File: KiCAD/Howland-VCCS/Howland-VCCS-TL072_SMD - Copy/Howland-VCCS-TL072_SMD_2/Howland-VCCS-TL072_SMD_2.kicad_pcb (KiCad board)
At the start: 2 copper layers, 24.5 x 25.4 mm, 16 parts, among them J1 Conn_01x03_Pin, J2 Conn_01x03_Pin, U1 TL072

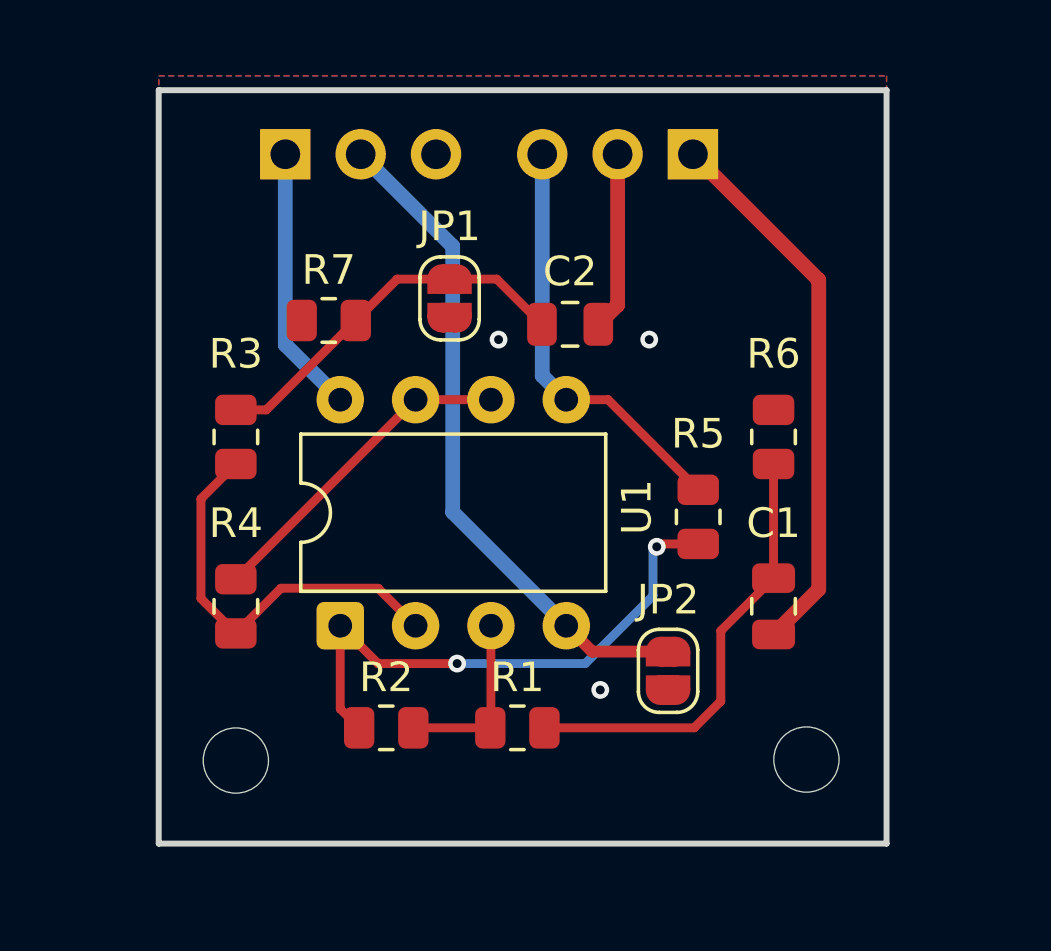
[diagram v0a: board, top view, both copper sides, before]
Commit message: Add Project Folder: KICAD
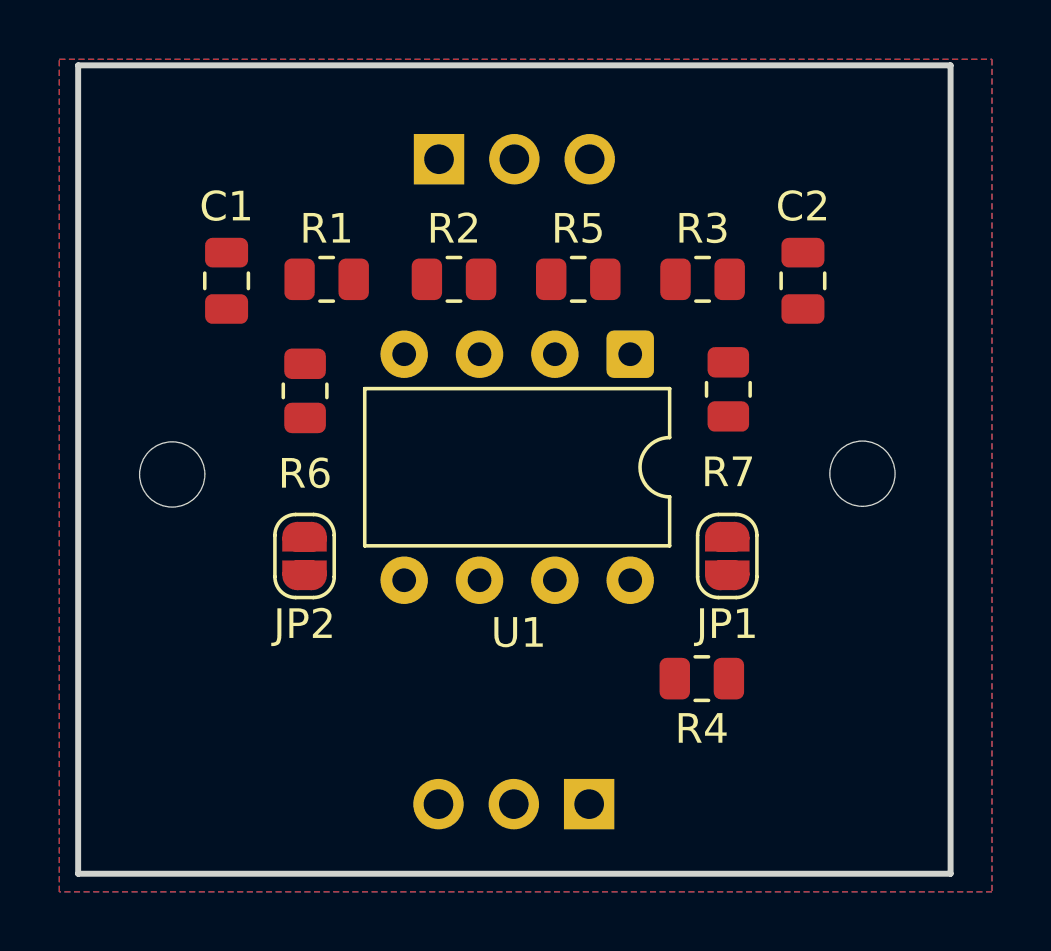
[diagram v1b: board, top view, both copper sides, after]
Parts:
- moved J2 24.2 mm to (192.4, 105.1), turned to 90 degrees
- moved C1 21.5 mm to (180.2, 87.4), turned to -90 degrees
- moved R3 16.6 mm to (196.2, 87.4), turned to 180 degrees
- moved R1 16.4 mm to (183.6, 87.4), turned to 0 degrees
- moved R4 15.9 mm to (196.2, 100.8), turned to 180 degrees
- moved R6 15.9 mm to (182.8, 91.1), turned to 90 degrees
- moved R2 15.3 mm to (187.9, 87.4), turned to 0 degrees
- moved R7 13.7 mm to (197.1, 91.1), turned to -90 degrees
- moved U1 13.4 mm to (193.8, 89.9), turned to -90 degrees
- moved JP2 12.9 mm to (182.8, 96.7)
- moved JP1 12.8 mm to (197.1, 96.7)
- moved H1 9.88 mm to (178.4, 94.0)
- moved H2 9.82 mm to (201.6, 93.9)
- moved R5 8.97 mm to (192.0, 87.4), turned to 0 degrees
- moved J1 8.56 mm to (187.4, 83.3), turned to -90 degrees
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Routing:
- net VEE: track 22.6 -> 0.00 mm
- net Net-(R2-Pad2): track 18.9 -> 0.00 mm, vias 2 -> 0
- net /Id+: track 18.6 -> 0.00 mm
- net Net-(C1-Pad2): track 15.1 -> 0.00 mm
- net /Out: track 14.3 -> 0.00 mm
- net Net-(U1A--): track 13.9 -> 0.00 mm
- net Net-(JP1-B): track 12.8 -> 0.00 mm
- net Net-(U1B--): track 11.1 -> 0.00 mm
- net VCC: track 9.04 -> 0.00 mm
- net Net-(U1A-+): track 6.05 -> 0.00 mm
- net /Id-: track 6.00 -> 0.00 mm
- net GND: vias 3 -> 0
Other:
- board size 24.5 x 25.4 mm -> 29.4 x 27.3 mm
